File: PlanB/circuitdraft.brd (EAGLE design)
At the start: 35 x 40 mm, 22 parts, among them Y1 CY16BPS

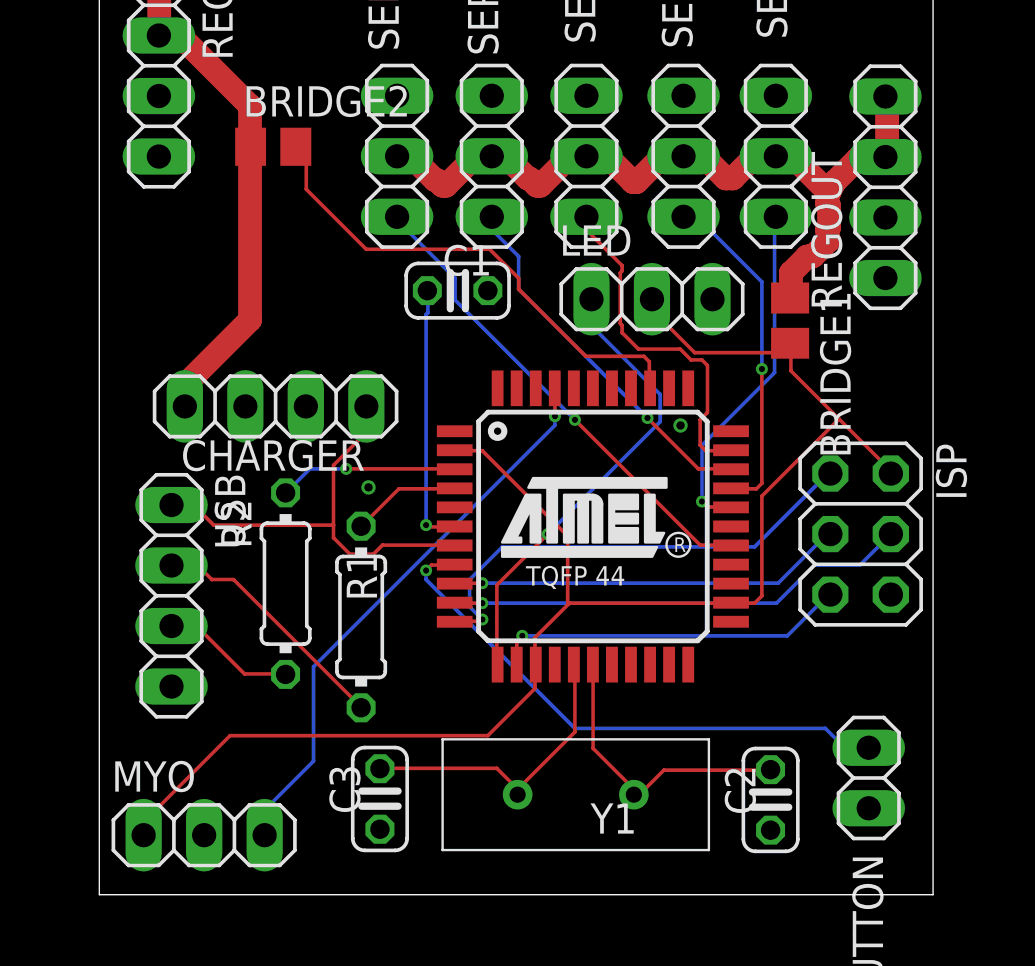
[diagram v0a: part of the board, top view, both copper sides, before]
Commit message: final refinement
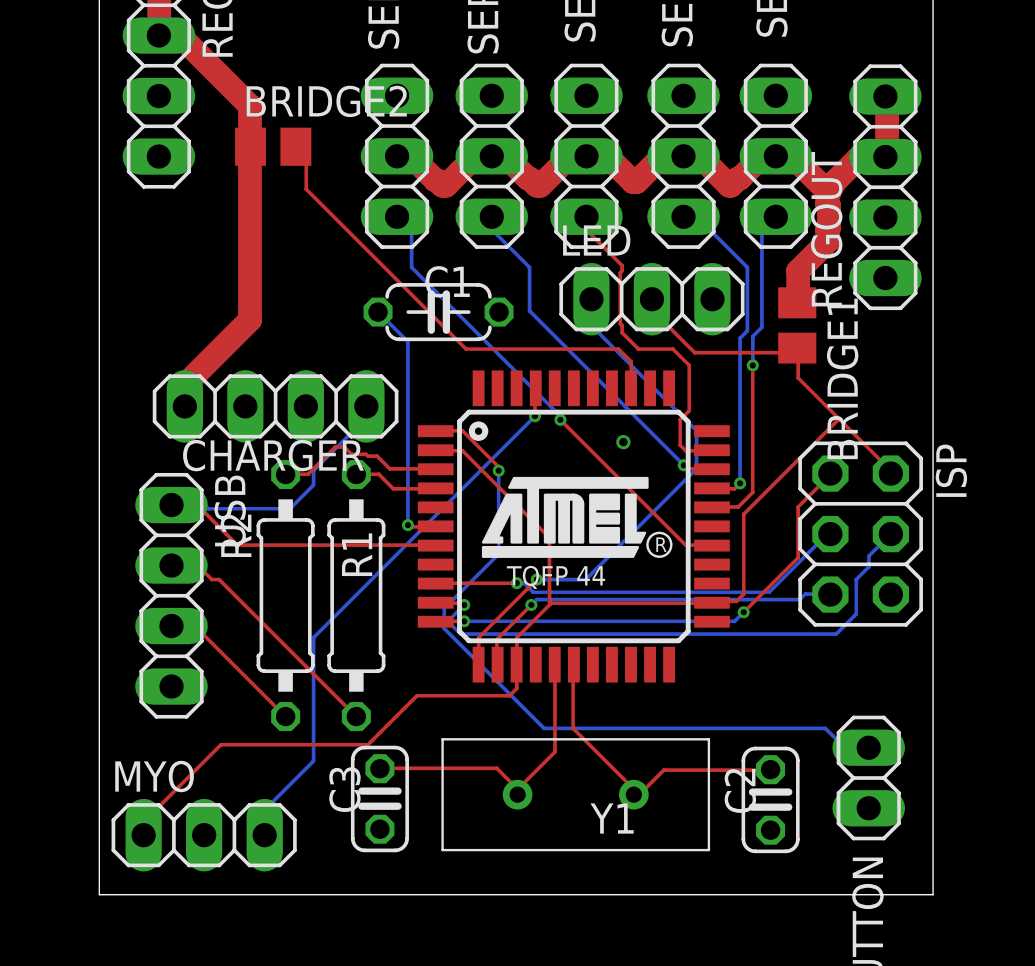
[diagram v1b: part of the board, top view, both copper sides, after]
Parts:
- C1: device rcl:C025-024X044 -> rcl:C050-024X044
- R1, R2: device rcl:0204/7 -> rcl:0207/10
- moved C1 1.20 mm to (22.2, 27.5)
- moved R1 0.92 mm to (18.8, 15.6)
- moved U$1 0.80 mm to (27.9, 18.5)
- moved R2 0.50 mm to (15.8, 15.6)
- moved BRIDGE1 0.36 mm to (37.3, 26.9)
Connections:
- net INTERRUPT: now also U$1.1; no longer U$1.8
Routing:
- net INTERRUPT: track 23.2 -> 30.9 mm
- net MOSI: track 19.5 -> 23.7 mm
- net VBUS: track 18.8 -> 22.5 mm
- net DATAIN: track 19.4 -> 22.2 mm
- net SCK: track 16.7 -> 17.8 mm
- net N$9: track 20.8 -> 19.7 mm
- net N$4: track 4.58 -> 3.59 mm
- net RST: track 15.0 -> 15.9 mm
- net POWER: track 64.3 -> 63.6 mm
- net D-: track 5.63 -> 6.37 mm
- net SIGNAL3: track 14.6 -> 13.9 mm
- net SIGNAL1: track 14.6 -> 13.9 mm
- net SIGNAL4: track 15.6 -> 15.0 mm
- net N$2: track 7.52 -> 7.16 mm, vias 1 -> 0
- net MISO: track 20.1 -> 20.4 mm, vias 1 -> 2
